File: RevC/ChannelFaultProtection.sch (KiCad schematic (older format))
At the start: 1 part

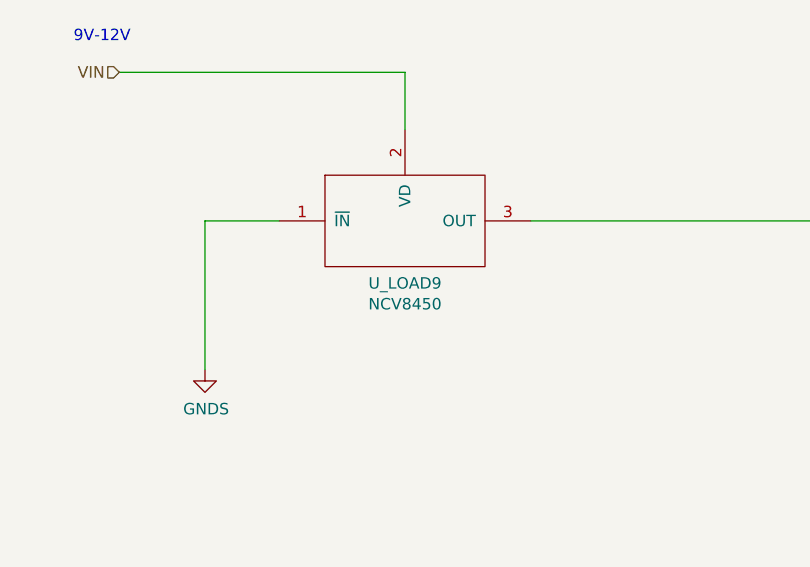
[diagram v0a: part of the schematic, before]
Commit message: updates
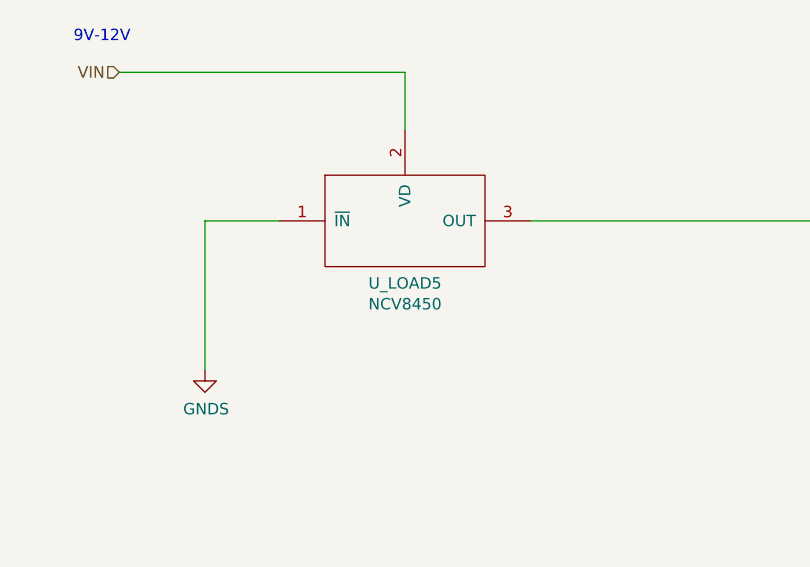
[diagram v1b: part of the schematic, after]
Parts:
- U_LOAD2: LcscNo (none) -> C100028
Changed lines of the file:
@@
 $Descr A4 11693 8268
 encoding utf-8
-Sheet 11 29
+Sheet 15 29
 Title ""
 Date ""
@@
 AR Path="/5DF46F3E/5DF57DA8" Ref="U_LOAD8"  Part="1"
 AR Path="/5DF61078/5DF57DA8" Ref="U_LOAD9"  Part="1"
-F 0 "U_LOAD9" H 5950 2677 50  0000 C CNN
+F 0 "U_LOAD5" H 5950 2677 50  0000 C CNN
 F 1 "NCV8450" H 5950 2586 50  0000 C CNN
 F 2 "Package_TO_SOT_SMD:SOT-223-3_TabPin2" H 5950 2700 50  0001 C CNN
-F 3 "" H 5950 3100 50  0001 C CNN
+F 3 "https://datasheet.lcsc.com/szlcsc/1912111437_ON-Semiconductor-NCV8450ASTT3G_C100028.pdf" H 5950 3100 50  0001 C CNN
+F 4 "C100028" H 5950 2950 50  0001 C CNN "LcscNo"
 	1    5950 2950
 	1    0    0    -1
